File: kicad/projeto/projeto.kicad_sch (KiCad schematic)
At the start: 43 parts, among them Q1 BTA16-600B, Q2 BTA16-600B, U1 ESP-12E, U3v3 LM1117-3.3

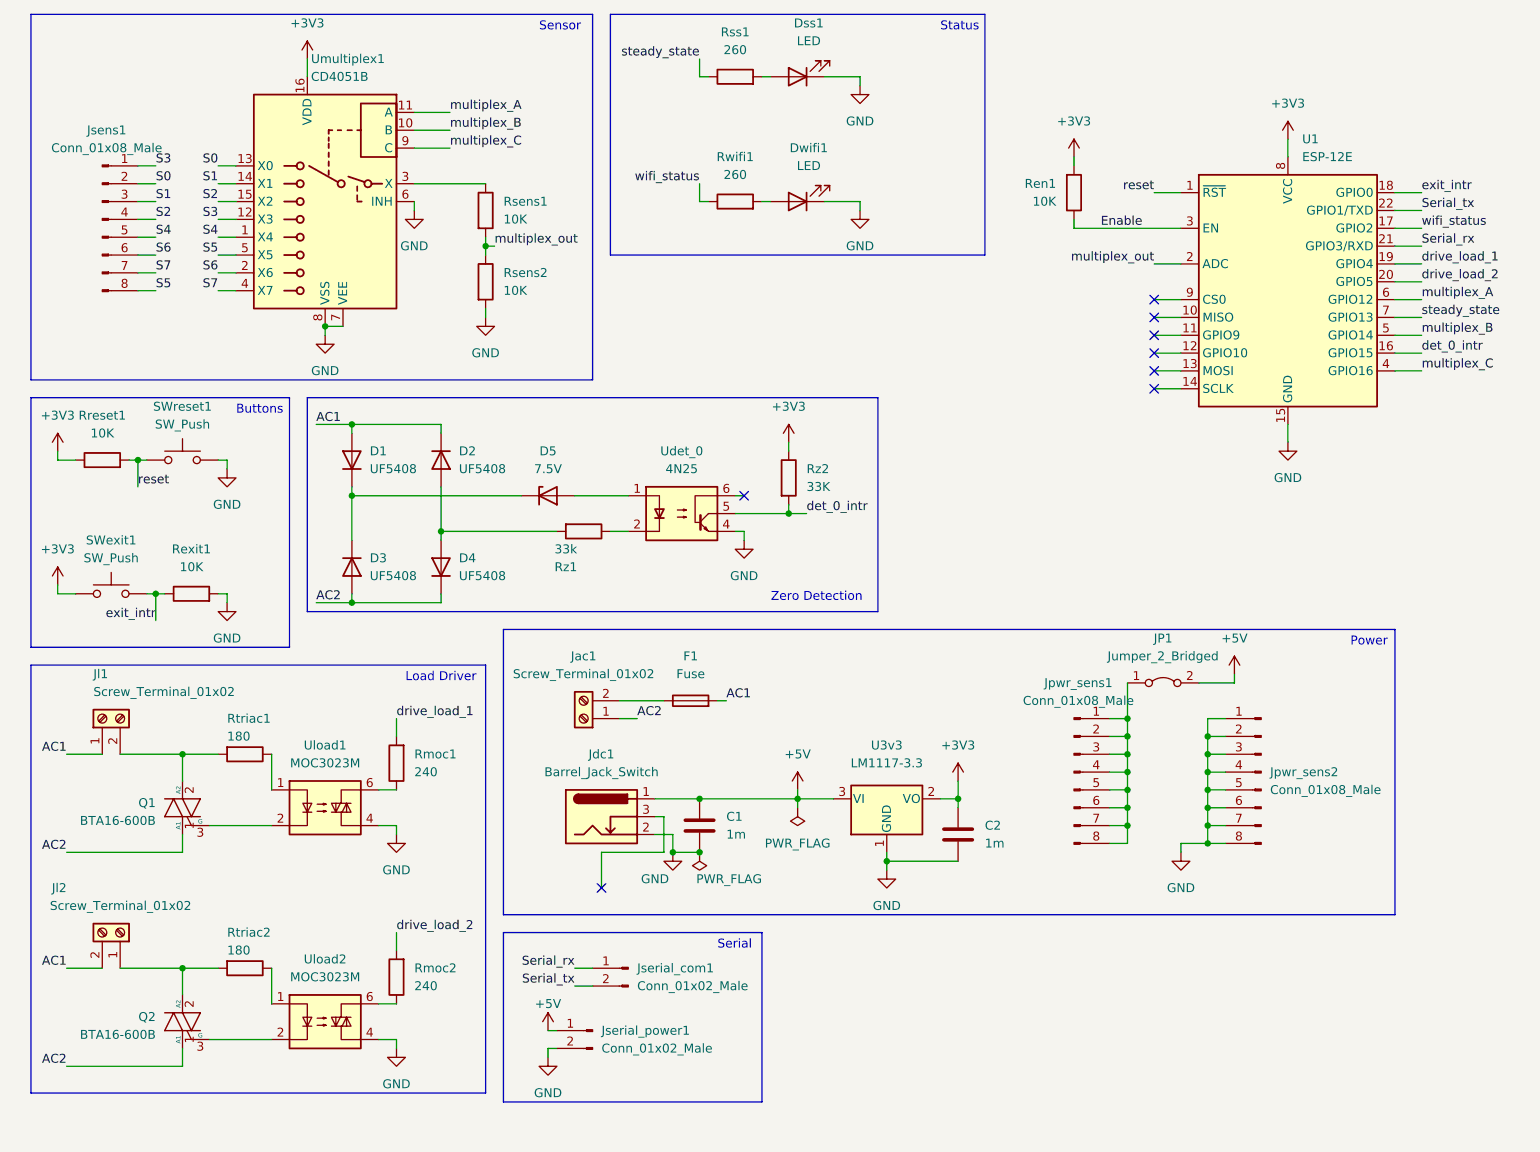
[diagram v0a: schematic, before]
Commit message: Fazendo a PCB
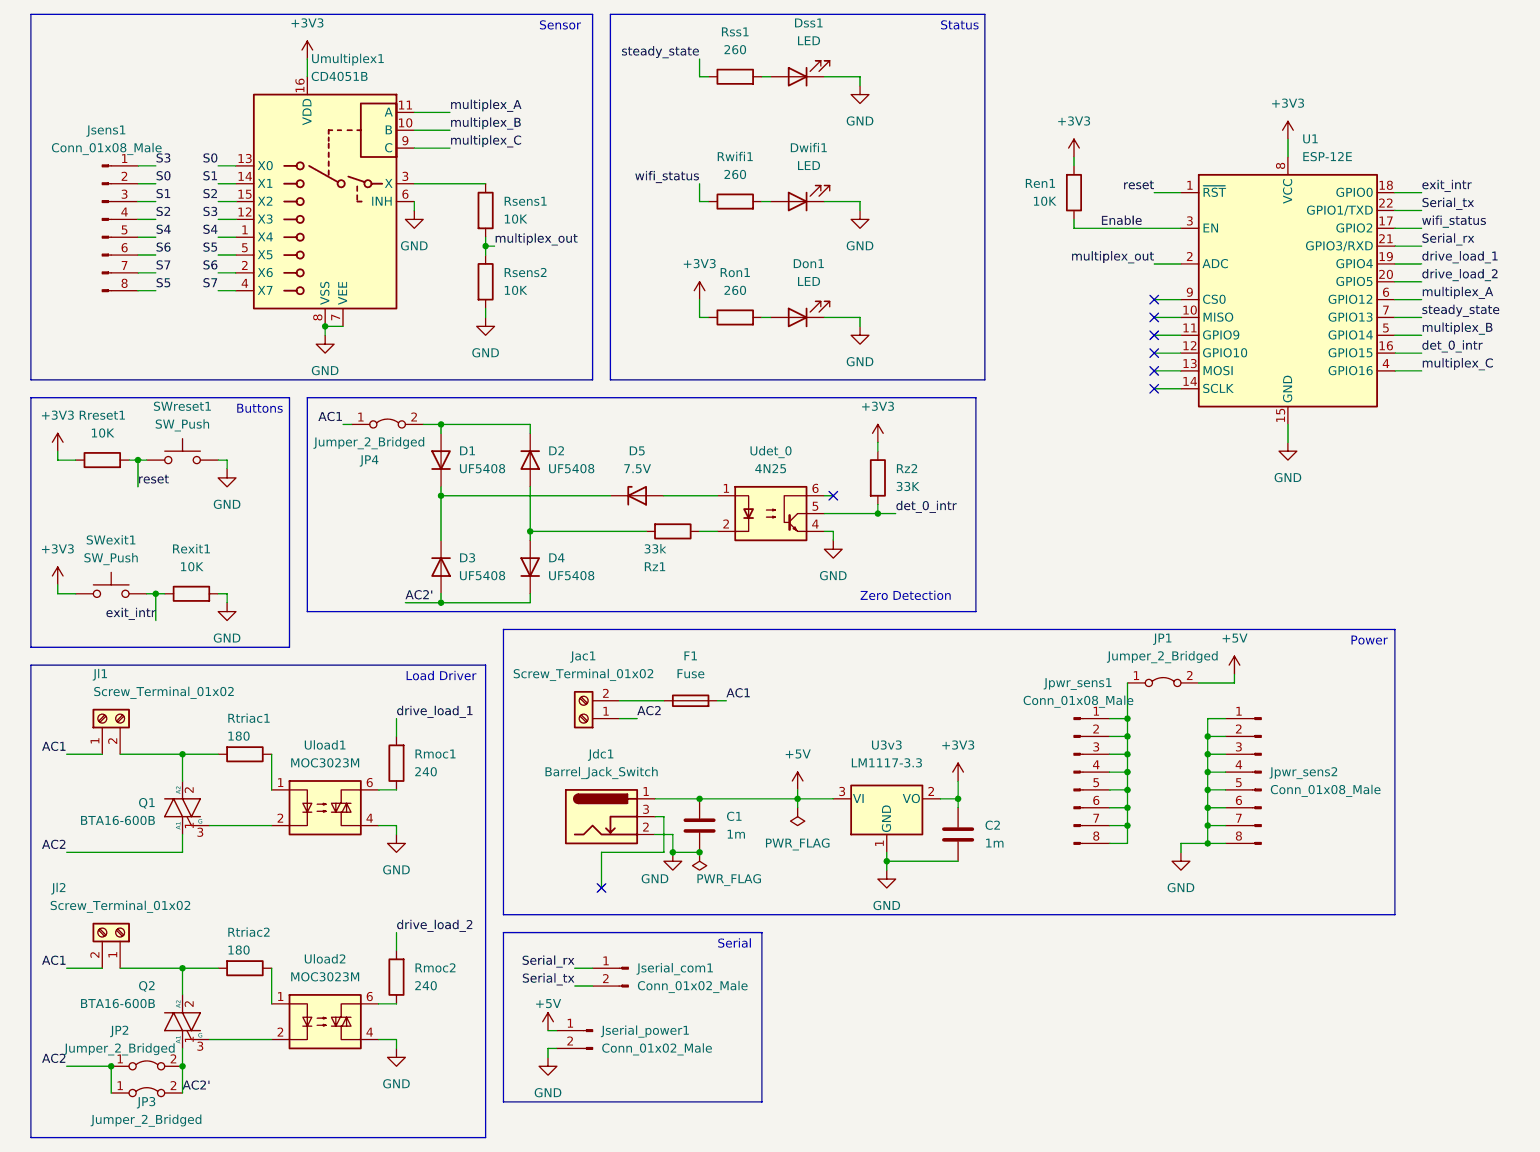
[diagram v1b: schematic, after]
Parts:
- added Don1: LED, LED_THT:LED_D3.0mm, symbol Device:LED
- added JP2, JP3, JP4: Jumper_2_Bridged, Jumper:jumper_10mm, symbol Jumper:Jumper_2_Bridged
- added Ron1: 260, Resistor_THT:R_Axial_DIN0207_L6.3mm_D2.5mm_P7.62mm_Horizontal, symbol Device:R
- Udet_0: footprint Package_DIP:DIP-6_W7.62mm -> Package_DIP:DIP-6_W7.62mm_Socket_LongPads
- Uload1, Uload2: footprint Package_DIP:DIP-6_W7.62mm_LongPads -> Package_DIP:DIP-6_W7.62mm_Socket_LongPads
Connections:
- net +3V3: now also Ron1.1
- net AC1: now also JP4.1 (A); no longer D1.2 (A), D2.1 (K)
- net AC2: now also JP2.1 (A), JP3.1 (A); no longer D3.2 (A), D4.1 (K), Q2.1 (A1)
- net GND: now also Don1.1 (K)
- new net: D1.2 (A), D2.1 (K), JP4.2 (B)
- new net: Don1.2 (A), Ron1.2
- new net AC2': D3.2 (A), D4.1 (K), JP2.2 (B), JP3.2 (B), Q2.1 (A1)
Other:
- moved on the sheet: D1, D2, D3, D4, D5, Rz1, Rz2, Udet_0
